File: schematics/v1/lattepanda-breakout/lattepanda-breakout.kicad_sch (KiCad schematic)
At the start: 26 parts, among them J1 Arduino, J2 Arduino, J3 COM(RS232/485), J4 Front Panel, J5 RS422, J6 RS485, J7 RS232, J8 PiKVM, J9 SDI12, SW1 3V3/5V, U1 MAX22508, U2 TRSF3232ECD, U3 MAX22508, U4 MAX22508

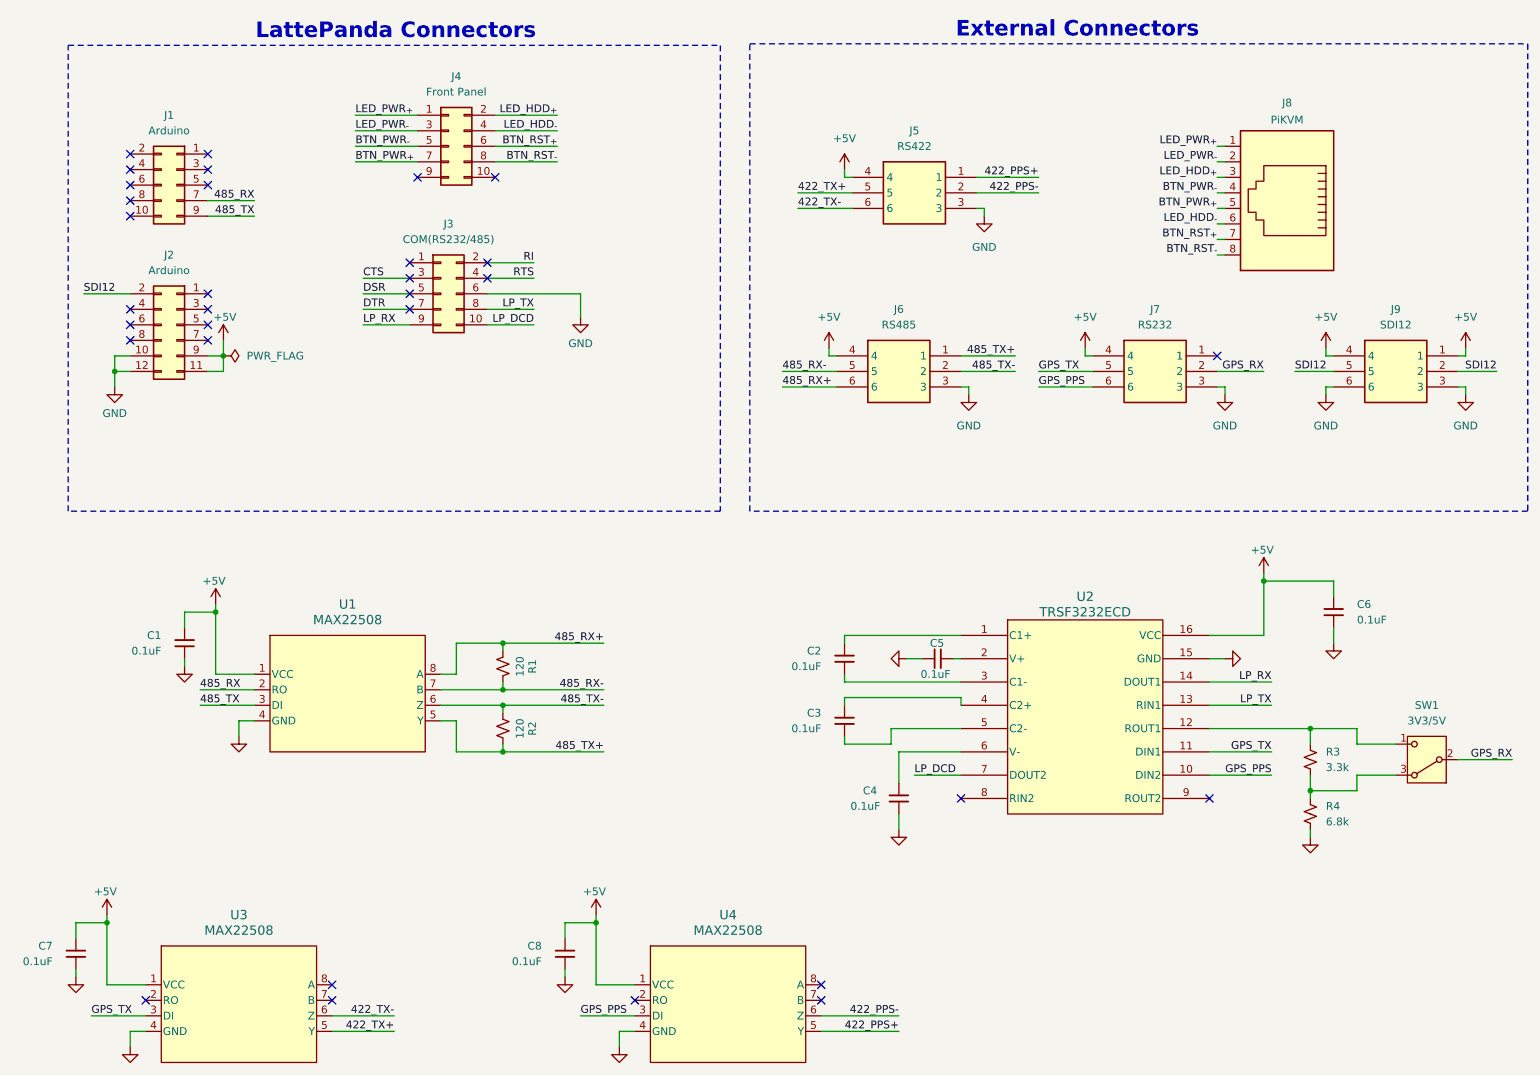
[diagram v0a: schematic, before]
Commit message: lattepanda-breakout finish
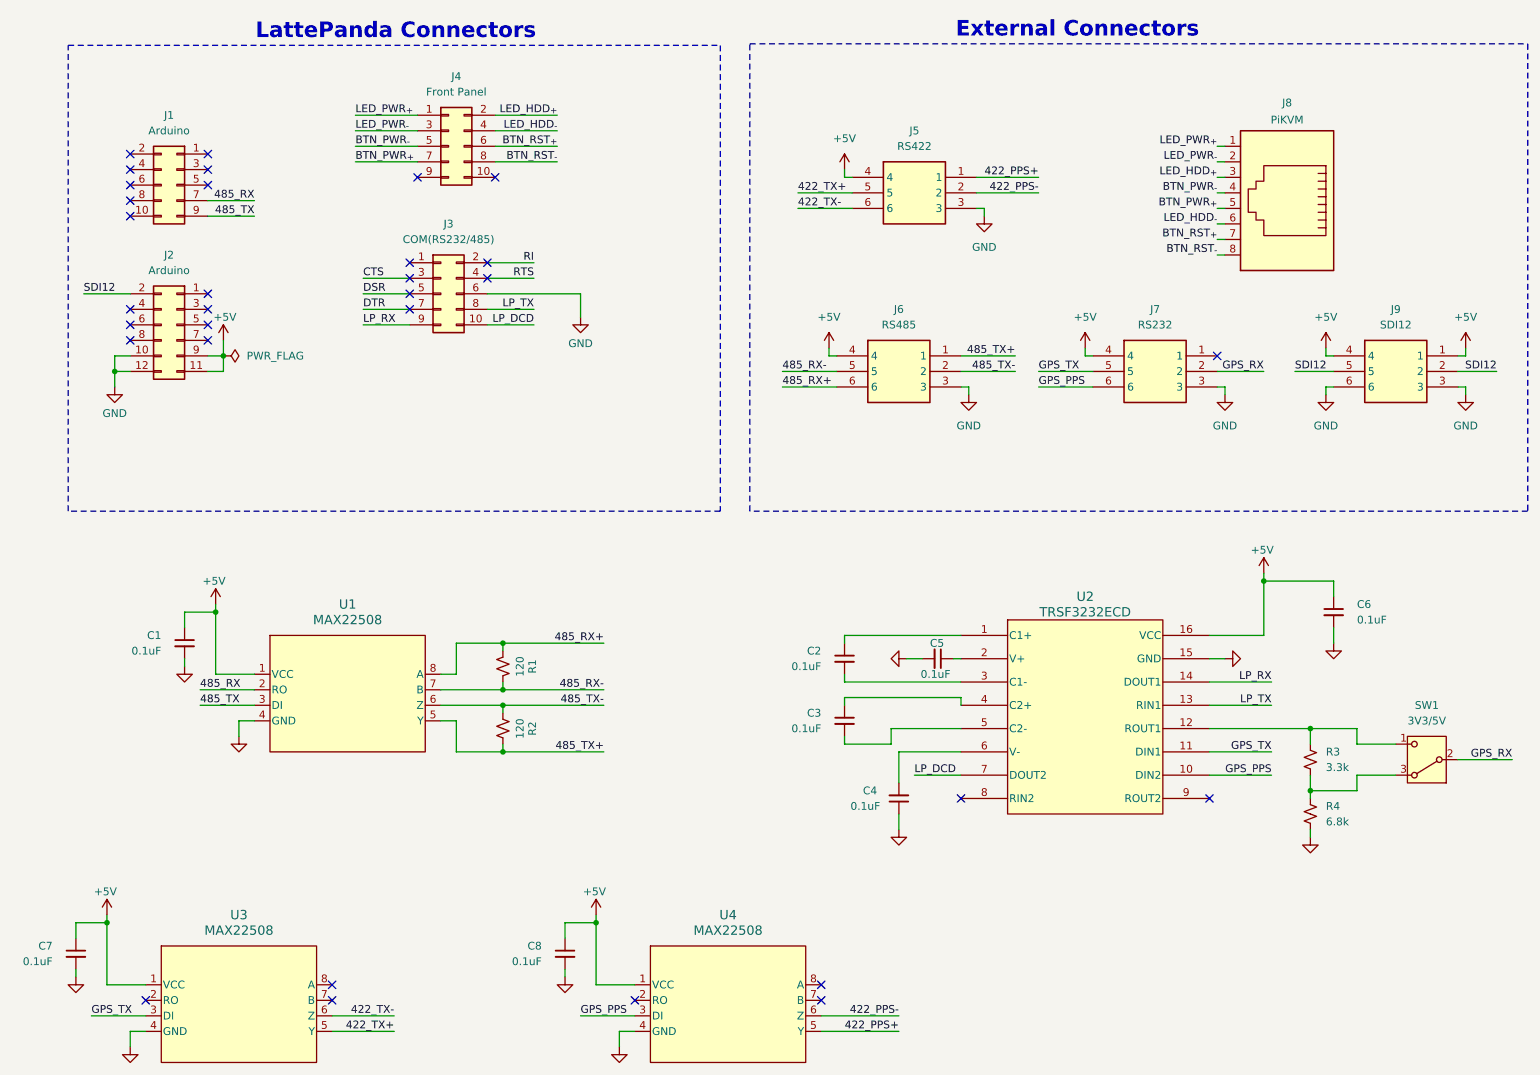
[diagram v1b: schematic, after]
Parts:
- C1, C2, C3, C4, C5, C6, C7, C8: MPN (none) -> C0603C104K5RACTU
- J1: MPN (none) -> 10129381-910004BLF
- J2: MPN (none) -> 10129381-912004BLF
- J3, J4: MPN (none) -> SSK04-FPH-254-B5
- J5: footprint Link_Footprints:PC-1053866 -> 1818517; MPN (none) -> 1818517; Manufacturer_Name Phoenix Contact -> (none); Manufacturer_Part_Number 1818517 -> (none); Mouser Part Number 651-1818517 -> (none); Mouser Price/Stock https://www.mouser.co.uk/ProductDetail/Phoenix-Contact/1818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 -> (none)
- J6, J7, J9: footprint Link_Footprints:PC-1053866 -> 1818517; MPN (none) -> 1818517; Manufacturer_Part_Number 1818517 -> (none); Mouser Part Number 651-1818517 -> (none); Mouser Price/Stock https://www.mouser.co.uk/ProductDetail/Phoenix-Contact/1818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 -> (none)
- J8: MPN (none) -> 1433900000
- R1, R2: MPN (none) -> RMEF0603JT120R
- R3: MPN (none) -> RMEF0603JT3K30
- R4: MPN (none) -> CRG0603F6K8
- SW1: symbol Switch:SW_Nidec_CAS-120A1 -> Link_Components:SW_Nidec_CAS-120A1; MPN (none) -> CAS-120TA
- U1, U3, U4: footprint Link_Footprints:MAX22508 -> 21-0041_S8+2C_MXM; MPN (none) -> MAX22508EASA+
- U2: footprint Link_Footprints:TRFS3232E -> D16; MPN (none) -> TRSF3232ECDR
